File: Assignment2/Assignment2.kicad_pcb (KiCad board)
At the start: 2 copper layers, 1 part, among them U1 RP2040

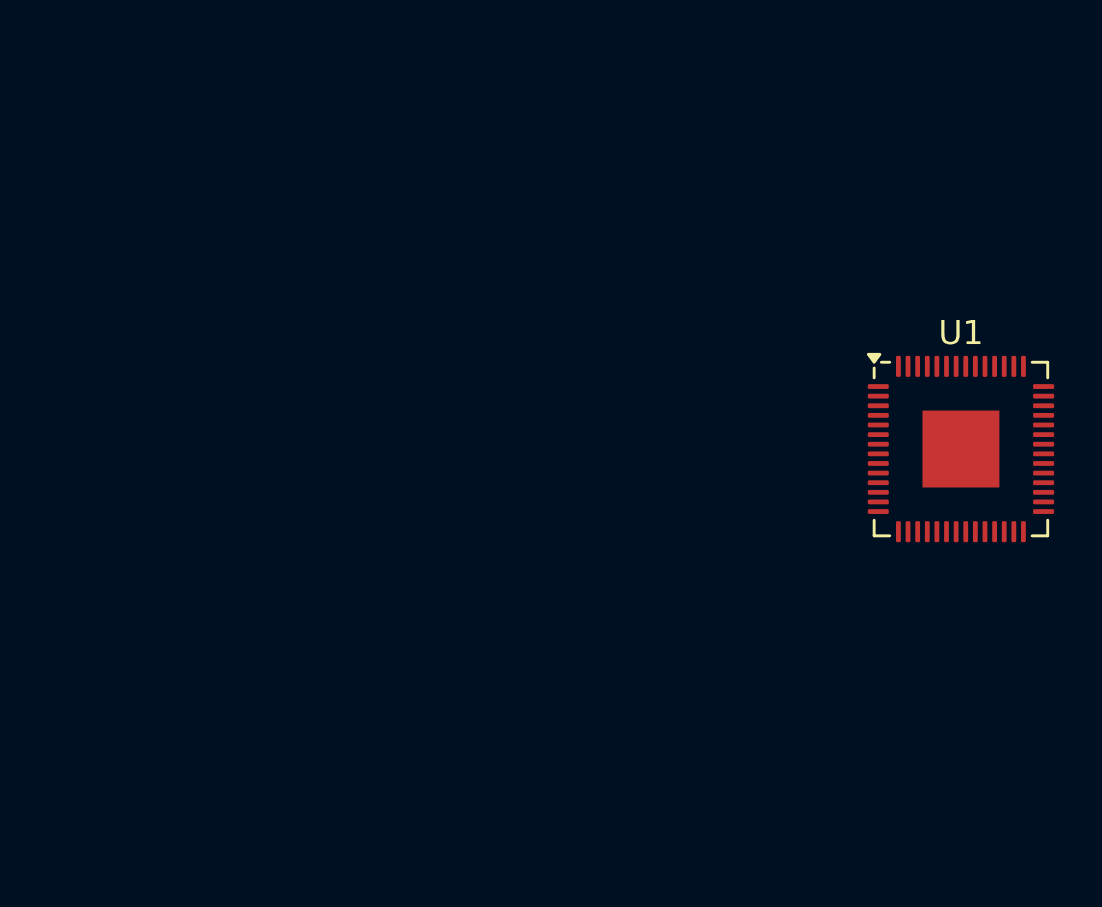
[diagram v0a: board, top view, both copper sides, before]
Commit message: assignment2: microphone and color module
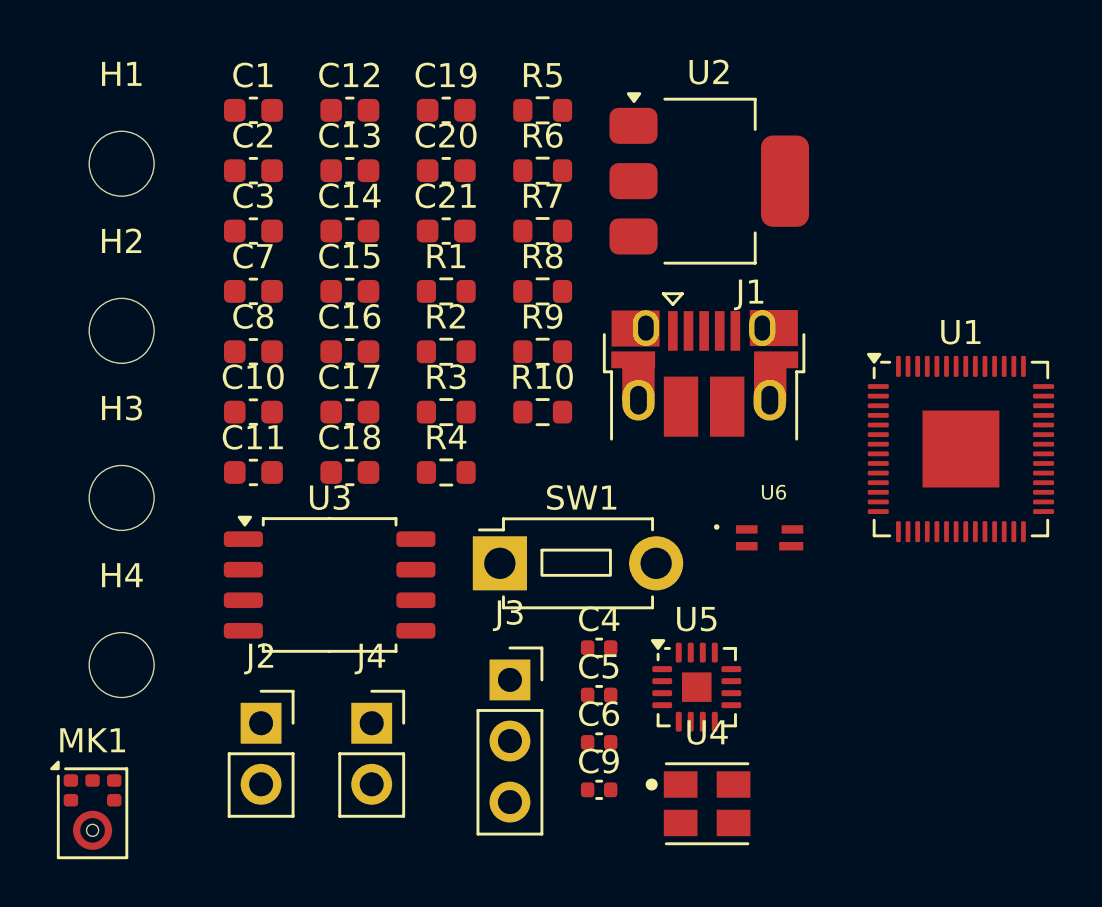
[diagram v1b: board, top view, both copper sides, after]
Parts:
- added C1: 10μF, Capacitor_SMD:C_0603_1608Metric, F.Cu at (106.5, 68.9)
- added C10: 100nF, Capacitor_SMD:C_0603_1608Metric, F.Cu at (106.5, 81.4)
- added C11: 100nF, Capacitor_SMD:C_0603_1608Metric, F.Cu at (106.5, 83.9)
- added C12: 100nF, Capacitor_SMD:C_0603_1608Metric, F.Cu at (110.5, 68.9)
- added C13: 100nF, Capacitor_SMD:C_0603_1608Metric, F.Cu at (110.5, 71.4)
- added C14: 100nF, Capacitor_SMD:C_0603_1608Metric, F.Cu at (110.5, 73.9)
- added C15: 100nF, Capacitor_SMD:C_0603_1608Metric, F.Cu at (110.5, 76.4)
- added C16: 100nF, Capacitor_SMD:C_0603_1608Metric, F.Cu at (110.5, 78.9)
- added C17: 10μF, Capacitor_SMD:C_0603_1608Metric, F.Cu at (110.5, 81.4)
- added C18: 0.1μF, Capacitor_SMD:C_0603_1608Metric, F.Cu at (110.5, 83.9)
- added C19: 0.1μF, Capacitor_SMD:C_0603_1608Metric, F.Cu at (114.6, 68.9)
- added C2: 10μF, Capacitor_SMD:C_0603_1608Metric, F.Cu at (106.5, 71.4)
- added C20: 200pF, Capacitor_SMD:C_0603_1608Metric, F.Cu at (114.6, 71.4)
- added C21: 100nF, Capacitor_SMD:C_0603_1608Metric, F.Cu at (114.6, 73.9)
- added C3: 100μF, Capacitor_SMD:C_0603_1608Metric, F.Cu at (106.5, 73.9)
- added C4: 15pF, Capacitor_SMD:C_0402_1005Metric, F.Cu at (120.9, 91.2)
- added C5: 15pF, Capacitor_SMD:C_0402_1005Metric, F.Cu at (120.9, 93.2)
- added C6: 1μF, Capacitor_SMD:C_0402_1005Metric, F.Cu at (120.9, 95.2)
- added C7: 100nF, Capacitor_SMD:C_0603_1608Metric, F.Cu at (106.5, 76.4)
- added C8: 100nF, Capacitor_SMD:C_0603_1608Metric, F.Cu at (106.5, 78.9)
- added C9: 1μF, Capacitor_SMD:C_0402_1005Metric, F.Cu at (120.9, 97.1)
- added H1: MountingHole, MountingHole:MountingHole_2.7mm_M2.5, F.Cu at (101.1, 71.1)
- added H2: MountingHole, MountingHole:MountingHole_2.7mm_M2.5, F.Cu at (101.1, 78.0)
- added H3: MountingHole, MountingHole:MountingHole_2.7mm_M2.5, F.Cu at (101.1, 85.0)
- added H4: MountingHole, MountingHole:MountingHole_2.7mm_M2.5, F.Cu at (101.1, 91.9)
- added J1: USB_B_Micro, Connector_USB:USB_Micro-B_Amphenol_10103594-0001LF_Horizontal, F.Cu at (125.3, 79.8)
- added J2: Conn_01x02, Connector_PinSocket_2.54mm:PinSocket_1x02_P2.54mm_Vertical, F.Cu at (106.9, 94.4)
- added J3: Conn_01x03, Connector_PinSocket_2.54mm:PinSocket_1x03_P2.54mm_Vertical, F.Cu at (117.2, 92.6)
- added J4: Conn_01x02, Connector_PinSocket_2.54mm:PinSocket_1x02_P2.54mm_Vertical, F.Cu at (111.5, 94.4)
- added MK1: SPH0645LM4H, Sensor_Audio:Knowles_SPH0645LM4H-6_3.5x2.65mm, F.Cu at (99.8, 98.1)
- added R1: 1kΩ, Resistor_SMD:R_0603_1608Metric, F.Cu at (114.6, 76.4)
- added R10: 2.2kΩ, Resistor_SMD:R_0603_1608Metric, F.Cu at (118.6, 81.4)
- added R2: DNF, Resistor_SMD:R_0603_1608Metric, F.Cu at (114.6, 78.9)
- added R3: 27Ω, Resistor_SMD:R_0603_1608Metric, F.Cu at (114.6, 81.4)
- added R4: 27Ω, Resistor_SMD:R_0603_1608Metric, F.Cu at (114.6, 83.9)
- added R5: 1MΩ, Resistor_SMD:R_0603_1608Metric, F.Cu at (118.6, 68.9)
- added R6: 51Ω, Resistor_SMD:R_0603_1608Metric, F.Cu at (118.6, 71.4)
- added R7: 51Ω, Resistor_SMD:R_0603_1608Metric, F.Cu at (118.6, 73.9)
- added R8: 51Ω, Resistor_SMD:R_0603_1608Metric, F.Cu at (118.6, 76.4)
- added R9: 2.2kΩ, Resistor_SMD:R_0603_1608Metric, F.Cu at (118.6, 78.9)
- added SW1: SW_Push, Button_Switch_THT:SW_PUSH_1P1T_6x3.5mm_H4.3_APEM_MJTP1243, F.Cu at (116.8, 87.7)
- added U2: NCP1117-3.3_SOT223, Package_TO_SOT_SMD:SOT-223-3_TabPin2, F.Cu at (125.5, 71.8)
- added U3: W25Q128JVS, Package_SO:SOIC-8_5.3x5.3mm_P1.27mm, F.Cu at (109.7, 88.6)
- added U4: ABM8-272-T3, ABM8-272-T3:ABM8-272-T3, F.Cu at (125.4, 97.7)
- added U5: MAX98357A, Package_DFN_QFN:TQFN-16-1EP_3x3mm_P0.5mm_EP1.23x1.23mm, F.Cu at (125.0, 92.9)
- added U6: VEML6040, VEML6040:VISHAY_VEML6040_1.25X2X1, F.Cu at (128.0, 86.6)
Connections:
- U1 pad 1: Net-(U1-IOVDD-Pad1) -> +3.3V
- U1 pad 10: Net-(U1-IOVDD-Pad1) -> +3.3V
- U1 pad 19: unconnected-(U1-TESTEN-Pad19) -> GND
- U1 pad 2: unconnected-(U1-GPIO0-Pad2) -> /GPIO0
- U1 pad 20: unconnected-(U1-XIN-Pad20) -> /XIN
- U1 pad 21: unconnected-(U1-XOUT-Pad21) -> /XOUT
- U1 pad 22: Net-(U1-IOVDD-Pad1) -> +3.3V
- U1 pad 23: Net-(U1-DVDD-Pad23) -> +1V1
- U1 pad 24: unconnected-(U1-SWCLK-Pad24) -> /SWCLK
- U1 pad 25: unconnected-(U1-SWD-Pad25) -> /SWD
- U1 pad 26: unconnected-(U1-RUN-Pad26) -> /RUN
- U1 pad 3: unconnected-(U1-GPIO1-Pad3) -> /GPIO1
- U1 pad 33: Net-(U1-IOVDD-Pad1) -> +3.3V
- U1 pad 4: unconnected-(U1-GPIO2-Pad4) -> /GPIO2
- U1 pad 42: Net-(U1-IOVDD-Pad1) -> +3.3V
- U1 pad 43: unconnected-(U1-ADC_AVDD-Pad43) -> +3.3V
- U1 pad 44: unconnected-(U1-VREG_IN-Pad44) -> +3.3V
- U1 pad 45: unconnected-(U1-VREG_VOUT-Pad45) -> +1V1
- U1 pad 46: unconnected-(U1-USB_DM-Pad46) -> Net-(U1-USB_DM)
- U1 pad 47: unconnected-(U1-USB_DP-Pad47) -> Net-(U1-USB_DP)
- U1 pad 48: unconnected-(U1-USB_VDD-Pad48) -> +3.3V
- U1 pad 49: Net-(U1-IOVDD-Pad1) -> +3.3V
- U1 pad 5: unconnected-(U1-GPIO3-Pad5) -> /GPIO3
- U1 pad 50: Net-(U1-DVDD-Pad23) -> +1V1
- U1 pad 51: unconnected-(U1-QSPI_SD3-Pad51) -> /QSPI_SD3
- U1 pad 52: unconnected-(U1-QSPI_SCLK-Pad52) -> /QSPI_SCLK
- U1 pad 53: unconnected-(U1-QSPI_SD0-Pad53) -> /QSPI_SD0
- U1 pad 54: unconnected-(U1-QSPI_SD2-Pad54) -> /QSPI_SD2
- U1 pad 55: unconnected-(U1-QSPI_SD1-Pad55) -> /QSPI_SD1
- U1 pad 56: unconnected-(U1-QSPI_SS-Pad56) -> /QSPI_SS
- U1 pad 57: unconnected-(U1-GND-Pad57) -> GND
- U1 pad 6: unconnected-(U1-GPIO4-Pad6) -> /GPIO4
- U1 pad 7: unconnected-(U1-GPIO5-Pad7) -> /GPIO5
- U1 pad 8: unconnected-(U1-GPIO6-Pad8) -> /GPIO6
- U1 pad 9: unconnected-(U1-GPIO7-Pad9) -> /GPIO7
